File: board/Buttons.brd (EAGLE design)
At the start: 50.5 x 21.6 mm, 4 parts

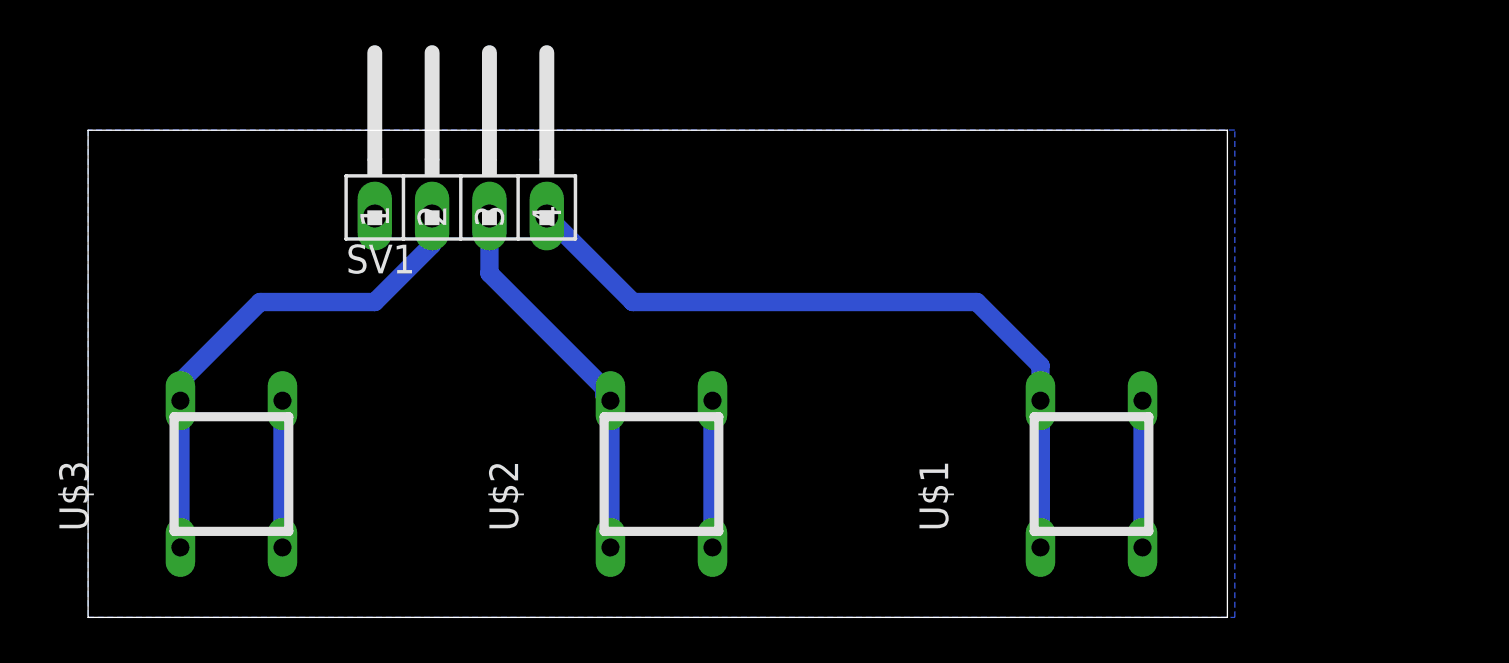
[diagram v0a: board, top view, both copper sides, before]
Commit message: Working on buttons board
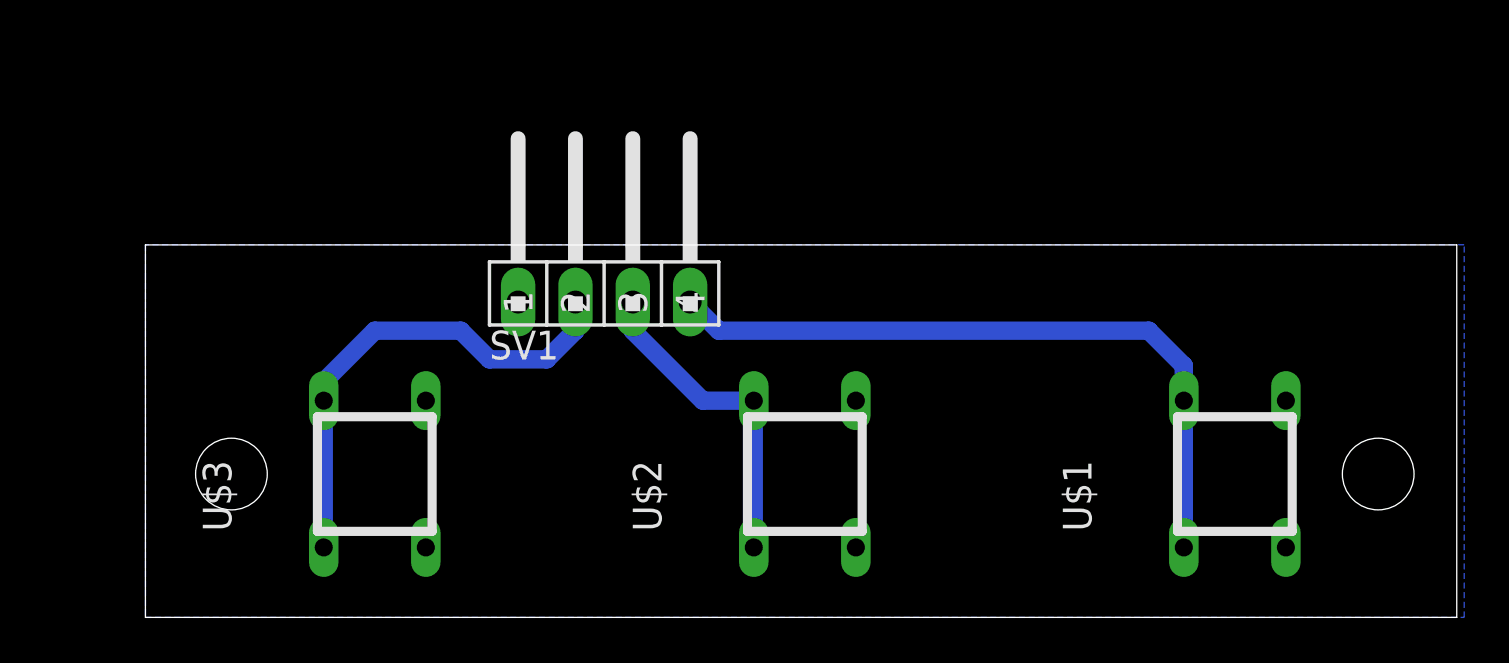
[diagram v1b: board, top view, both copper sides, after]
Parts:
- moved SV1 7.41 mm to (22.9, 14.0)
- moved U$2 6.35 mm to (31.8, 6.35)
- moved U$3 6.35 mm to (12.7, 6.35)
- moved U$1 6.35 mm to (50.8, 6.35)
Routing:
- net GND: track 19.5 -> 0.00 mm
- net N$3: track 39.2 -> 31.1 mm
- net N$2: track 17.6 -> 14.4 mm
- net N$1: track 22.3 -> 21.7 mm
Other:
- board size 50.5 x 21.6 mm -> 58.1 x 16.5 mm
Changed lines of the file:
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@@
 <layer number="43" name="vRestrict" color="2" fill="10" visible="yes" active="yes"/>
 <layer number="44" name="Drills" color="7" fill="1" visible="no" active="yes"/>
-<layer number="45" name="Holes" color="7" fill="1" visible="no" active="yes"/>
+<layer number="45" name="Holes" color="7" fill="1" visible="yes" active="yes"/>
 <layer number="46" name="Milling" color="3" fill="1" visible="no" active="yes"/>
 <layer number="47" name="Measures" color="7" fill="1" visible="no" active="yes"/>
@@
 <board>
 <plain>
-<wire x1="0" y1="0" x2="50.47" y2="0" width="0" layer="20"/>
-<wire x1="50.47" y1="0" x2="50.47" y2="21.58" width="0" layer="20"/>
-<wire x1="50.47" y1="21.58" x2="0" y2="21.58" width="0" layer="20"/>
-<wire x1="0" y1="21.58" x2="0" y2="0" width="0" layer="20"/>
+<wire x1="2.54" y1="0" x2="60.63" y2="0" width="0" layer="20"/>
+<wire x1="60.63" y1="0" x2="60.63" y2="16.5" width="0" layer="20"/>
+<wire x1="60.63" y1="16.5" x2="2.54" y2="16.5" width="0" layer="20"/>
+<wire x1="2.54" y1="16.5" x2="2.54" y2="0" width="0" layer="20"/>
+<hole x="6.35" y="6.35" drill="3.175"/>
+<hole x="57.15" y="6.35" drill="3.175"/>
 </plain>
 <attributes>
@@
 </autorouter>
 <elements>
-<element name="U$1" library="SuperFeed" package="PUSH" value="PUSH" x="44.45" y="6.35" rot="R90"/>
-<element name="U$2" library="SuperFeed" package="PUSH" value="PUSH" x="25.4" y="6.35" rot="R90"/>
-<element name="U$3" library="SuperFeed" package="PUSH" value="PUSH" x="6.35" y="6.35" rot="R90"/>
-<element name="SV1" library="SuperFeed" package="MA04-1W" value="" x="16.51" y="17.78"/>
+<element name="U$1" library="SuperFeed" package="PUSH" value="PUSH" x="50.8" y="6.35" rot="R90"/>
+<element name="U$2" library="SuperFeed" package="PUSH" value="PUSH" x="31.75" y="6.35" rot="R90"/>
+<element name="U$3" library="SuperFeed" package="PUSH" value="PUSH" x="12.7" y="6.35" rot="R90"/>
+<element name="SV1" library="SuperFeed" package="MA04-1W" value="" x="22.86" y="13.97"/>
 </elements>
 <signals>
@@
 <contactref element="U$3" pad="1"/>
 <contactref element="SV1" pad="2"/>
-<wire x1="4.0894" y1="3.0988" x2="4.0894" y2="9.6012" width="0.8128" layer="16"/>
-<wire x1="4.0894" y1="9.6012" x2="4.0894" y2="10.4394" width="0.8128" layer="16"/>
-<wire x1="4.0894" y1="10.4394" x2="7.62" y2="13.97" width="0.8128" layer="16"/>
-<wire x1="7.62" y1="13.97" x2="12.7" y2="13.97" width="0.8128" layer="16"/>
-<wire x1="12.7" y1="13.97" x2="15.24" y2="16.51" width="0.8128" layer="16"/>
-<wire x1="15.24" y1="16.51" x2="15.24" y2="17.78" width="0.8128" layer="16"/>
+<wire x1="10.4394" y1="3.0988" x2="10.4394" y2="9.6012" width="0.8128" layer="16"/>
+<wire x1="10.4394" y1="9.6012" x2="10.4394" y2="10.4394" width="0.8128" layer="16"/>
+<wire x1="10.4394" y1="10.4394" x2="12.7" y2="12.7" width="0.8128" layer="16"/>
+<wire x1="12.7" y1="12.7" x2="16.51" y2="12.7" width="0.8128" layer="16"/>
+<wire x1="16.51" y1="12.7" x2="17.78" y2="11.43" width="0.8128" layer="16"/>
+<wire x1="17.78" y1="11.43" x2="20.32" y2="11.43" width="0.8128" layer="16"/>
+<wire x1="20.32" y1="11.43" x2="21.59" y2="12.7" width="0.8128" layer="16"/>
+<wire x1="21.59" y1="12.7" x2="21.59" y2="13.97" width="0.8128" layer="16"/>
 </signal>
 <signal name="N$3">
@@
 <contactref element="U$1" pad="1"/>
 <contactref element="SV1" pad="4"/>
-<wire x1="42.1894" y1="3.0988" x2="42.1894" y2="9.6012" width="0.8128" layer="16"/>
-<wire x1="42.1894" y1="3.0988" x2="42.1894" y2="11.1506" width="0.8128" layer="16"/>
-<wire x1="42.1894" y1="11.1506" x2="39.37" y2="13.97" width="0.8128" layer="16"/>
-<wire x1="39.37" y1="13.97" x2="24.13" y2="13.97" width="0.8128" layer="16"/>
-<wire x1="24.13" y1="13.97" x2="20.32" y2="17.78" width="0.8128" layer="16"/>
+<wire x1="48.5394" y1="3.0988" x2="48.5394" y2="9.6012" width="0.8128" layer="16"/>
+<wire x1="48.5394" y1="9.6012" x2="48.5394" y2="11.1506" width="0.8128" layer="16"/>
+<wire x1="48.5394" y1="11.1506" x2="46.99" y2="12.7" width="0.8128" layer="16"/>
+<wire x1="46.99" y1="12.7" x2="27.94" y2="12.7" width="0.8128" layer="16"/>
+<wire x1="27.94" y1="12.7" x2="26.67" y2="13.97" width="0.8128" layer="16"/>
 </signal>
 <signal name="GND">
@@
 <contactref element="U$3" pad="3"/>
 <contactref element="SV1" pad="1"/>
-<wire x1="8.6106" y1="3.0988" x2="8.6106" y2="9.6012" width="0.8128" layer="16"/>
-<wire x1="27.6606" y1="3.0988" x2="27.6606" y2="9.6012" width="0.8128" layer="16"/>
-<wire x1="46.7106" y1="9.6012" x2="46.7106" y2="3.0988" width="0.8128" layer="16"/>
 <polygon width="0.8128" layer="16">
-<vertex x="0" y="0"/>
-<vertex x="50.8" y="0"/>
-<vertex x="50.8" y="21.59"/>
-<vertex x="0" y="21.59"/>
+<vertex x="2.54" y="0"/>
+<vertex x="60.96" y="0"/>
+<vertex x="60.96" y="16.51"/>
+<vertex x="2.54" y="16.51"/>
 </polygon>
 </signal>
@@
 <contactref element="U$2" pad="1"/>
 <contactref element="SV1" pad="3"/>
-<wire x1="23.1394" y1="3.0988" x2="23.1394" y2="9.6012" width="0.8128" layer="16"/>
-<wire x1="23.1394" y1="9.6012" x2="23.1394" y2="9.8806" width="0.8128" layer="16"/>
-<wire x1="23.1394" y1="9.8806" x2="22.86" y2="10.16" width="0.8128" layer="16"/>
-<wire x1="22.86" y1="10.16" x2="22.86" y2="9.8806" width="0.8128" layer="16"/>
-<wire x1="22.86" y1="9.8806" x2="23.1394" y2="9.6012" width="0.8128" layer="16"/>
-<wire x1="17.78" y1="17.78" x2="17.78" y2="15.24" width="0.8128" layer="16"/>
-<wire x1="17.78" y1="15.24" x2="22.86" y2="10.16" width="0.8128" layer="16"/>
+<wire x1="29.4894" y1="9.6012" x2="27.2288" y2="9.6012" width="0.8128" layer="16"/>
+<wire x1="27.2288" y1="9.6012" x2="24.13" y2="12.7" width="0.8128" layer="16"/>
+<wire x1="24.13" y1="12.7" x2="24.13" y2="13.97" width="0.8128" layer="16"/>
+<wire x1="29.4894" y1="9.6012" x2="29.4894" y2="3.0988" width="0.8128" layer="16"/>
 </signal>
 </signals>
